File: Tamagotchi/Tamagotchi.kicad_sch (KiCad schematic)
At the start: 2 parts, among them U1 XIAO-ESP32-C6-DIP, U2 DM-OLED096-636

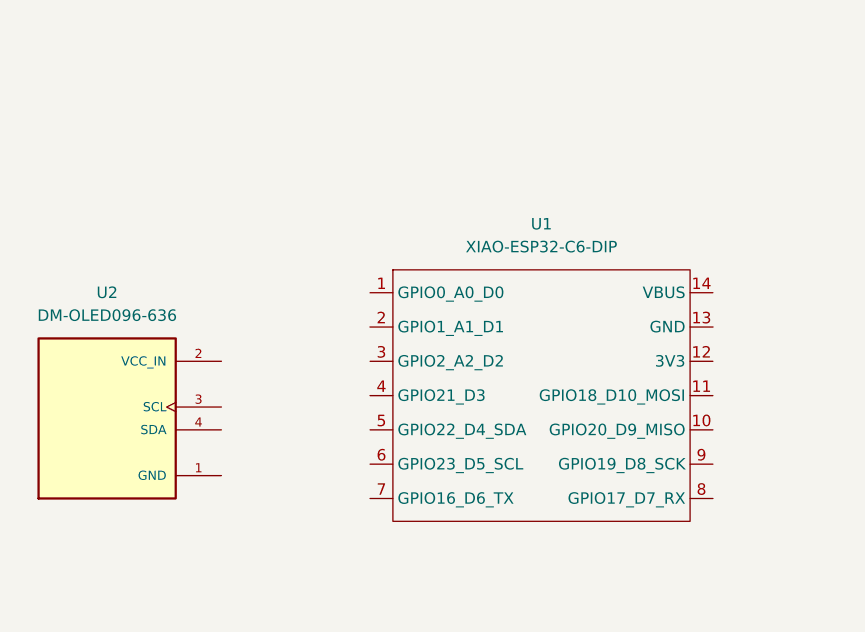
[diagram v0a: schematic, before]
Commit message: finished the schematic
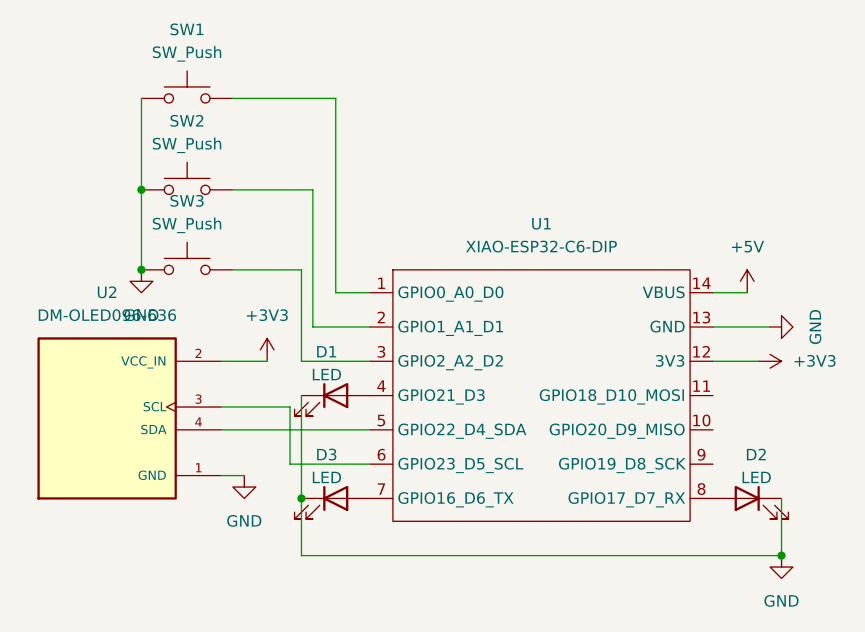
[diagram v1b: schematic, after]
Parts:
- added D1, D2, D3: LED, LED_THT:LED_D1.8mm_W1.8mm_H2.4mm_Horizontal_O1.27mm_Z4.9mm, symbol Device:LED
- added SW1, SW2, SW3: SW_Push, Button_Switch_THT:KSA_Tactile_SPST, symbol Switch:SW_Push
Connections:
- net GND: now reaches U2.1 (GND)
- net GND: now also U1.13 (GND), D1.1 (K), D2.1 (K), D3.1 (K), SW1.1, SW2.1, SW3.1
- net +3V3: now reaches U2.2 (VCC_IN)
- net +3V3: now also U1.12 (3V3)
- net at U2.3 (SCL): now also U1.6 (GPIO23_D5_SCL)
- net at U2.4 (SDA): now also U1.5 (GPIO22_D4_SDA)
- net at U1.1 (GPIO0_A0_D0): now also SW1.2
- net +5V: now reaches U1.14 (VBUS)
- net at U1.2 (GPIO1_A1_D1): now also SW2.2
- net at U1.3 (GPIO2_A2_D2): now also SW3.2
- net at U1.4 (GPIO21_D3): now also D1.2 (A)
- net at U1.7 (GPIO16_D6_TX): now also D3.2 (A)
- net at U1.8 (GPIO17_D7_RX): now also D2.2 (A)
